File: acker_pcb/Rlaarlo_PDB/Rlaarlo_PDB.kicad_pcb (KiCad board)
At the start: 2 copper layers, 88.2 x 108.4 mm, 9 parts, among them J1 xt 60, J2 Conn_01x03_Pin, J3 Conn_01x02_Pin, SW1 SW_SPST, SW2 SW_SPST, SW3 SW_SPST

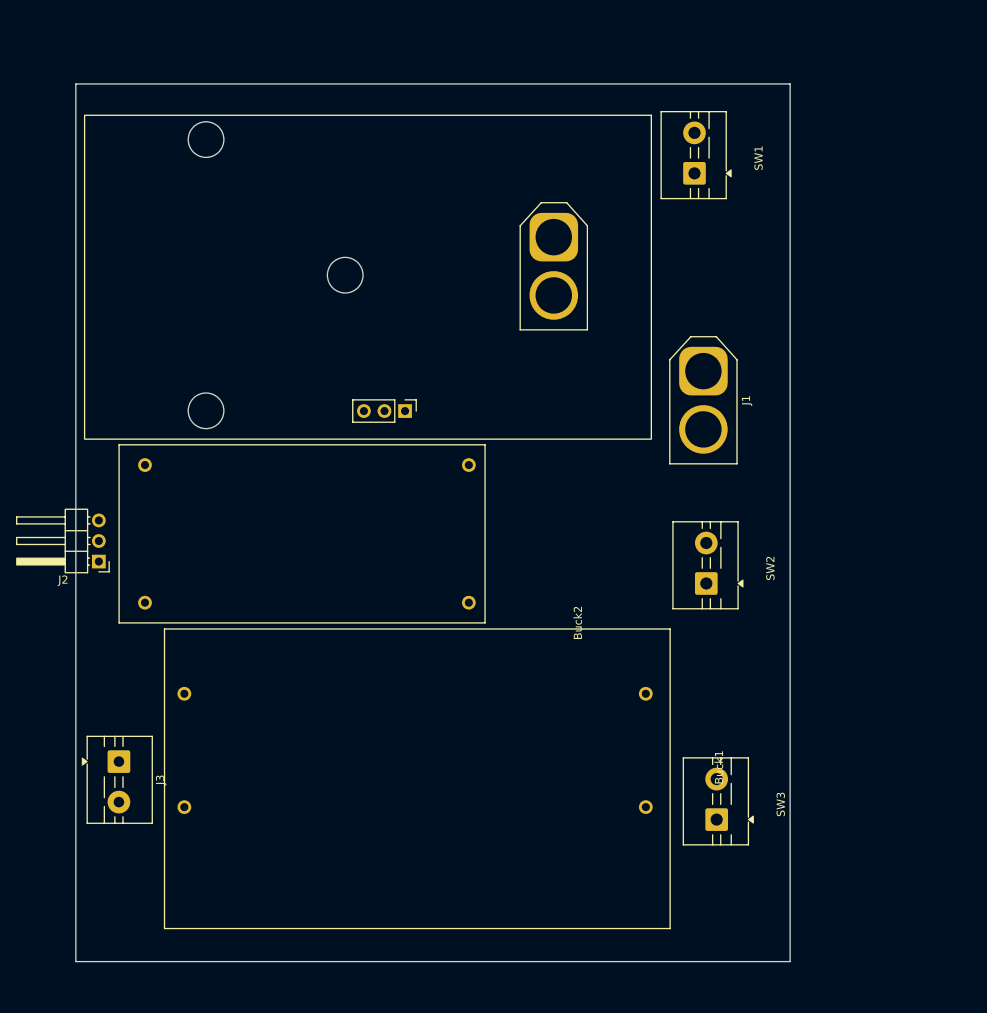
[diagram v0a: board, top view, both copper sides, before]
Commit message: pcb updates
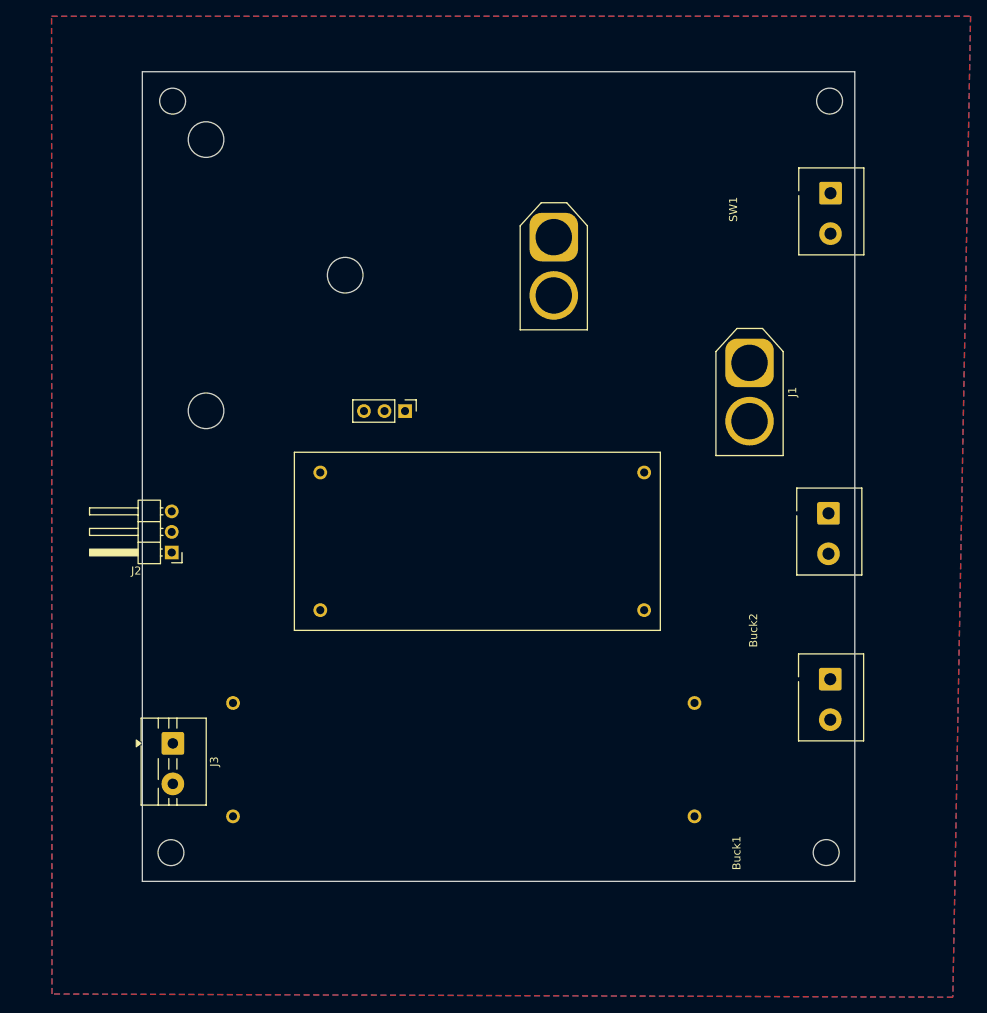
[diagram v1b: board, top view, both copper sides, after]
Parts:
- added REF**: MountingHole_3.2mm_M3, MountingHole:MountingHole_3.2mm_M3, F.Cu at (154.5, 121.4)
- added REF**: MountingHole_3.2mm_M3, MountingHole:MountingHole_3.2mm_M3, F.Cu at (154.9, 28.6)
- added REF**: MountingHole_3.2mm_M3, MountingHole:MountingHole_3.2mm_M3, F.Cu at (73.7, 28.6)
- added REF**: MountingHole_3.2mm_M3, MountingHole:MountingHole_3.2mm_M3, F.Cu at (73.5, 121.5)
- SW1: value SW_SPST -> SW_SPST_esb
- moved SW3 22.3 mm to (155.0, 100.0), turned to -90 degrees
- moved Buck2 21.7 mm to (134.0, 94.0)
- moved SW2 17.7 mm to (155.0, 79.3), turned to -90 degrees
- moved SW1 17.0 mm to (155.0, 40.0), turned to -90 degrees
- moved J2 9.07 mm to (73.6, 84.4)
- moved J3 7.03 mm to (73.8, 108.0)
- moved Buck1 6.12 mm to (141.2, 132.0)
- moved J1 5.79 mm to (145.0, 61.0)
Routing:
- added copper zone on B.Cu, net GND
- added copper zone on F.Cu, net GND
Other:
- board size 88.2 x 108.4 mm -> 88 x 100 mm
